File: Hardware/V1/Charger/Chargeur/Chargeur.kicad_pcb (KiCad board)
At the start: 2 copper layers, 50 x 40 mm, 30 parts, among them J1 USB_C_Receptacle_PowerOnly_6P, U1 LTC4125

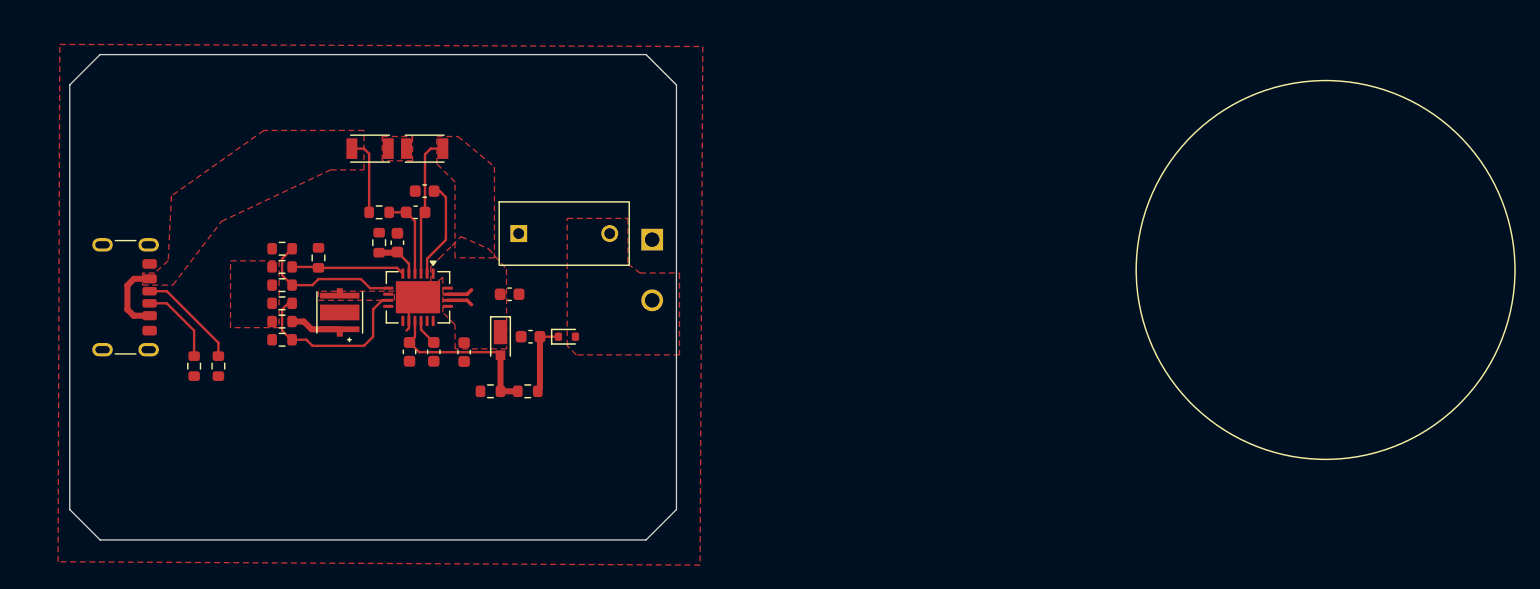
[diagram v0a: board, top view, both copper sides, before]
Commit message: Ibom charger
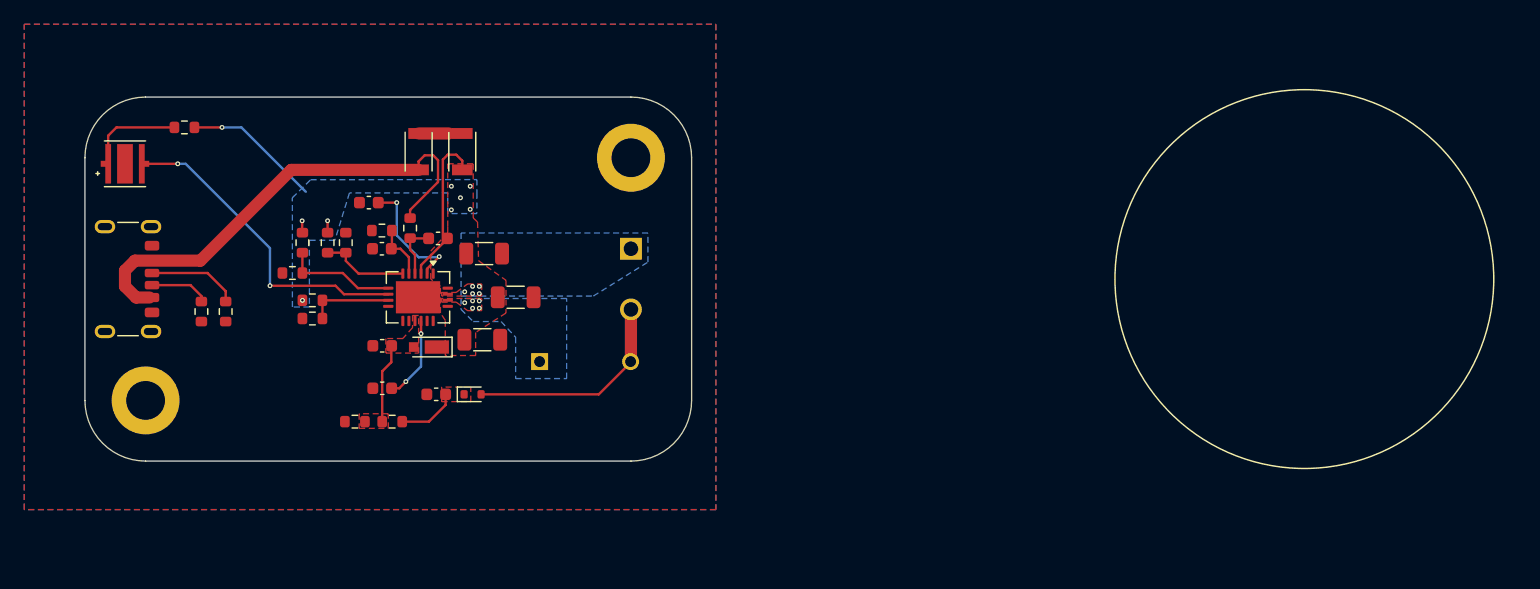
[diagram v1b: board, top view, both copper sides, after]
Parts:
- added C9: 1u, Capacitor_SMD:C_1206_3216Metric, F.Cu at (142.9, 82.9)
- added G***: LOGO, LOGO, B.Cu at (134.2, 85.0)
- added H1: MountingHole_Pad, MountingHole:MountingHole_3.2mm_M3_DIN965_Pad, F.Cu at (155.0, 75.0)
- added H2: MountingHole_Pad, MountingHole:MountingHole_3.2mm_M3_DIN965_Pad, F.Cu at (115.0, 95.0)
- C7, C8: footprint Capacitor_SMD:C_0603_1608Metric -> Capacitor_SMD:C_1206_3216Metric
- moved D3 21.5 mm to (113.3, 75.5), turned to 180 degrees
- moved R11 17.9 mm to (118.2, 72.5), turned to 0 degrees
- moved R1 11.5 mm to (135.3, 96.8)
- moved R2 11.5 mm to (132.2, 96.8)
- moved C0 10.7 mm to (147.5, 91.8)
- moved C2 9.11 mm to (138.9, 94.5)
- moved D2 9.11 mm to (141.9, 94.5)
- moved D1 6.14 mm to (138.1, 90.6), turned to 180 degrees
- moved C4 5.20 mm to (134.5, 94.0), turned to 180 degrees
- moved C3 4.70 mm to (133.4, 78.7)
- moved R12 4.54 mm to (121.6, 87.7)
- moved R15 4.54 mm to (119.6, 87.7)
- moved R4 4.25 mm to (130.0, 82.0), turned to 90 degrees
- moved R13 4.01 mm to (137.5, 74.5), turned to 90 degrees
- moved R9 3.88 mm to (127.9, 82.0), turned to 90 degrees
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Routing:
- net VCC: track 12.5 -> 40.1 mm
- net Net-(D3--): track 0.00 -> 26.6 mm, vias 0 -> 2
- net Net-(D2-A): track 0.00 -> 21.9 mm
- net +5V: track 11.6 -> 26.1 mm, vias 0 -> 9
- net Net-(U1-FTH): track 14.9 -> 6.93 mm
- net Net-(D1-A): track 14.2 -> 6.71 mm
- net Net-(U1-CTD): track 2.21 -> 6.92 mm, vias 0 -> 2
- net Net-(D3-+): track 4.19 -> 8.06 mm
- net GND: track 3.14 -> 0.00 mm
- net Net-(U1-DTH): track 12.1 -> 9.22 mm
- net Net-(R13-Pad2): track 0.00 -> 2.50 mm
- net Net-(U1-CTS): track 8.12 -> 10.3 mm, vias 0 -> 2
- net Net-(U1-IS+): track 6.75 -> 4.63 mm
- net Net-(U1-SW2): track 2.11 -> 0.00 mm, vias 0 -> 5
- net Net-(U1-SW1): track 2.11 -> 0.00 mm, vias 0 -> 5
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- added copper zone on B.Cu, net +5V
- added copper zone on B.Cu, net GND
- added copper zone on F.Cu, net Net-(D1-A)
- added copper zone on F.Cu, net Net-(D2-K)
- added copper zone on B.Cu, net Net-(U1-SW1)
- added copper zone on F.Cu, net Net-(U1-SW1)
- added copper zone on B.Cu, net Net-(U1-SW2)
- added copper zone on F.Cu, net Net-(U1-SW2)
- removed copper zone on F.Cu, net Net-(D2-A)
- removed copper zone on F.Cu, net Net-(D3--)
- removed copper zone on F.Cu, net Net-(R13-Pad2)
- removed copper zone on F.Cu, net VCC
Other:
- board size 50 x 40 mm -> 50 x 30 mm
